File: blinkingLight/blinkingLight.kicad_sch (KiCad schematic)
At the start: 11 parts, among them J1 Conn_02x03_Odd_Even, J2 Conn_01x02_Pin, Q1 BC548, U1 ICM7555xB

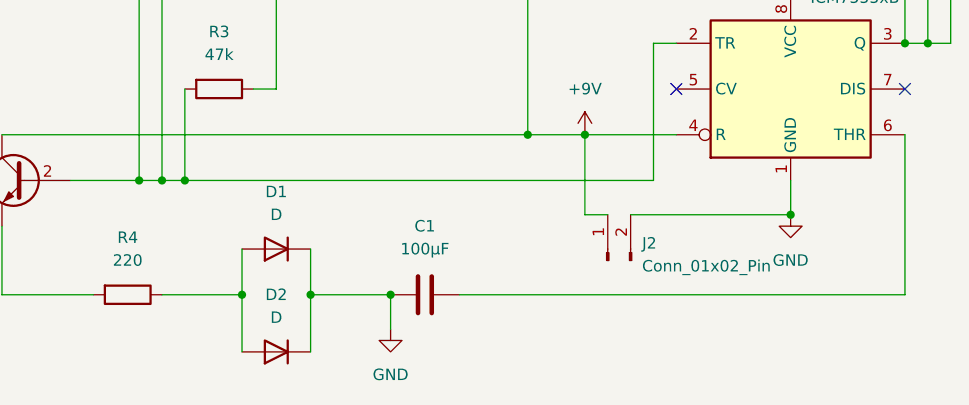
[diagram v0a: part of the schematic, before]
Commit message: push
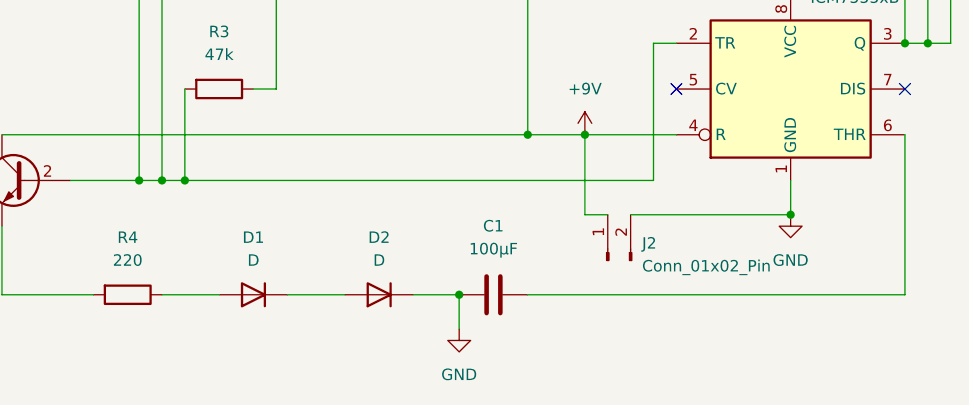
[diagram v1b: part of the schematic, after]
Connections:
- net GND: no longer D1.1 (K)
- net at D1.2 (A), R4.1: no longer D2.2 (A)
- new net: D1.1 (K), D2.2 (A)
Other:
- moved on the sheet: C1, D1, D2
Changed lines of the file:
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@@
 	)
 	(junction
-		(at 96.52 111.76)
-		(diameter 0)
-		(color 0 0 0 0)
-	)
-	(junction
-		(at 104.14 111.76)
+		(at 120.65 111.76)
 		(diameter 0)
 		(color 0 0 0 0)
@@
 	)
 	(junction
-		(at 113.03 111.76)
-		(diameter 0)
-		(color 0 0 0 0)
-	)
-	(junction
 		(at 157.48 102.87)
 		(diameter 0)
@@
 	(wire
 		(pts
-			(xy 104.14 111.76) (xy 104.14 118.11)
-		)
-		(stroke
-			(width 0)
-			(type default)
-		)
-	)
-	(wire
-		(pts
 			(xy 80.01 111.76) (xy 69.85 111.76)
 		)
@@
 	(wire
 		(pts
-			(xy 104.14 111.76) (xy 113.03 111.76)
-		)
-		(stroke
-			(width 0)
-			(type default)
-		)
-	)
-	(wire
-		(pts
 			(xy 77.47 99.06) (xy 85.09 99.06)
 		)
@@
 	(wire
 		(pts
+			(xy 87.63 111.76) (xy 93.98 111.76)
+		)
+		(stroke
+			(width 0)
+			(type default)
+		)
+	)
+	(wire
+		(pts
 			(xy 134.62 102.87) (xy 134.62 93.98)
 		)
@@
 	(wire
 		(pts
-			(xy 96.52 106.68) (xy 96.52 111.76)
+			(xy 115.57 111.76) (xy 120.65 111.76)
 		)
 		(stroke
@@
 	(wire
 		(pts
-			(xy 120.65 111.76) (xy 170.18 111.76)
+			(xy 128.27 111.76) (xy 170.18 111.76)
 		)
 		(stroke
@@
 	(wire
 		(pts
-			(xy 96.52 111.76) (xy 96.52 118.11)
-		)
-		(stroke
-			(width 0)
-			(type default)
-		)
-	)
-	(wire
-		(pts
 			(xy 172.72 69.85) (xy 172.72 83.82)
 		)
@@
 	(wire
 		(pts
-			(xy 113.03 111.76) (xy 113.03 115.57)
+			(xy 120.65 111.76) (xy 120.65 115.57)
+		)
+		(stroke
+			(width 0)
+			(type default)
+		)
+	)
+	(wire
+		(pts
+			(xy 101.6 111.76) (xy 107.95 111.76)
 		)
 		(stroke
@@
 	(wire
 		(pts
-			(xy 96.52 111.76) (xy 87.63 111.76)
-		)
-		(stroke
-			(width 0)
-			(type default)
-		)
-	)
-	(wire
-		(pts
 			(xy 90.17 67.31) (xy 85.09 67.31)
 		)
@@
 		(pts
 			(xy 69.85 111.76) (xy 69.85 104.14)
-		)
-		(stroke
-			(width 0)
-			(type default)
-		)
-	)
-	(wire
-		(pts
-			(xy 104.14 106.68) (xy 104.14 111.76)
 		)
 		(stroke
@@
 	(symbol
 		(lib_id "Device:C")
-		(at 116.84 111.76 270)
+		(at 124.46 111.76 270)
 		(unit 1)
 		(exclude_from_sim no)
@@
 		(fields_autoplaced yes)
 		(property "Reference" "C1"
-			(at 116.84 104.14 90)
+			(at 124.46 104.14 90)
 			(effects
 				(font
@@
 		)
 		(property "Value" "100μF"
-			(at 116.84 106.68 90)
+			(at 124.46 106.68 90)
 			(effects
 				(font
@@
 		)
 		(property "Footprint" "Capacitor_THT:CP_Radial_D8.0mm_P5.00mm"
-			(at 113.03 112.7252 0)
+			(at 120.65 112.7252 0)
 			(effects
 				(font
@@
 		)
 		(property "Datasheet" "~"
-			(at 116.84 111.76 0)
+			(at 124.46 111.76 0)
 			(effects
 				(font
@@
 		)
 		(property "Description" "Unpolarized capacitor"
-			(at 116.84 111.76 0)
+			(at 124.46 111.76 0)
 			(effects
 				(font
@@
 	(symbol
 		(lib_id "Device:D")
-		(at 100.33 118.11 180)
+		(at 111.76 111.76 180)
 		(unit 1)
 		(exclude_from_sim no)
@@
 		(fields_autoplaced yes)
 		(property "Reference" "D2"
-			(at 100.33 111.76 0)
+			(at 111.76 105.41 0)
 			(effects
 				(font
@@
 		)
 		(property "Value" "D"
-			(at 100.33 114.3 0)
+			(at 111.76 107.95 0)
 			(effects
 				(font
@@
 		)
 		(property "Footprint" "LED_THT:LED_D3.0mm_Horizontal_O6.35mm_Z10.0mm"
-			(at 100.33 118.11 0)
+			(at 111.76 111.76 0)
 			(effects
 				(font
@@
 		)
 		(property "Datasheet" "~"
-			(at 100.33 118.11 0)
+			(at 111.76 111.76 0)
 			(effects
 				(font
@@
 		)
 		(property "Description" "Diode"
-			(at 100.33 118.11 0)
+			(at 111.76 111.76 0)
 			(effects
 				(font
@@
 		)
 		(property "Sim.Device" "D"
-			(at 100.33 118.11 0)
+			(at 111.76 111.76 0)
 			(effects
 				(font
@@
 		)
 		(property "Sim.Pins" "1=K 2=A"
-			(at 100.33 118.11 0)
+			(at 111.76 111.76 0)
 			(effects
 				(font
@@
 	(symbol
 		(lib_id "power:GND")
-		(at 113.03 115.57 0)
+		(at 120.65 115.57 0)
 		(unit 1)
 		(exclude_from_sim no)
@@
 		(fields_autoplaced yes)
 		(property "Reference" "#PWR03"
-			(at 113.03 121.92 0)
+			(at 120.65 121.92 0)
 			(effects
 				(font
@@
 		)
 		(property "Value" "GND"
-			(at 113.03 120.65 0)
+			(at 120.65 120.65 0)
 			(effects
 				(font
@@
 		)
 		(property "Footprint" ""
-			(at 113.03 115.57 0)
+			(at 120.65 115.57 0)
 			(effects
 				(font
@@
 		)
 		(property "Datasheet" ""
-			(at 113.03 115.57 0)
+			(at 120.65 115.57 0)
 			(effects
 				(font
@@
 		)
 		(property "Description" "Power symbol creates a global label with name \"GND\" , ground"
-			(at 113.03 115.57 0)
+			(at 120.65 115.57 0)
 			(effects
 				(font
@@
 	(symbol
 		(lib_id "Device:D")
-		(at 100.33 106.68 180)
+		(at 97.79 111.76 180)
 		(unit 1)
 		(exclude_from_sim no)
@@
 		(fields_autoplaced yes)
 		(property "Reference" "D1"
-			(at 100.33 100.33 0)
+			(at 97.79 105.41 0)
 			(effects
 				(font
@@
 		)
 		(property "Value" "D"
-			(at 100.33 102.87 0)
+			(at 97.79 107.95 0)
 			(effects
 				(font
@@
 		)
 		(property "Footprint" "LED_THT:LED_D3.0mm_Horizontal_O6.35mm_Z10.0mm"
-			(at 100.33 106.68 0)
+			(at 97.79 111.76 0)
 			(effects
 				(font
@@
 		)
 		(property "Datasheet" "~"
-			(at 100.33 106.68 0)
+			(at 97.79 111.76 0)
 			(effects
 				(font
@@
 		)
 		(property "Description" "Diode"
-			(at 100.33 106.68 0)
+			(at 97.79 111.76 0)
 			(effects
 				(font
@@
 		)
 		(property "Sim.Device" "D"
-			(at 100.33 106.68 0)
+			(at 97.79 111.76 0)
 			(effects
 				(font
@@
 		)
 		(property "Sim.Pins" "1=K 2=A"
-			(at 100.33 106.68 0)
-			(effects
-				(font
+			(at 97.79 111.76 0)
+			(effects
+				(font

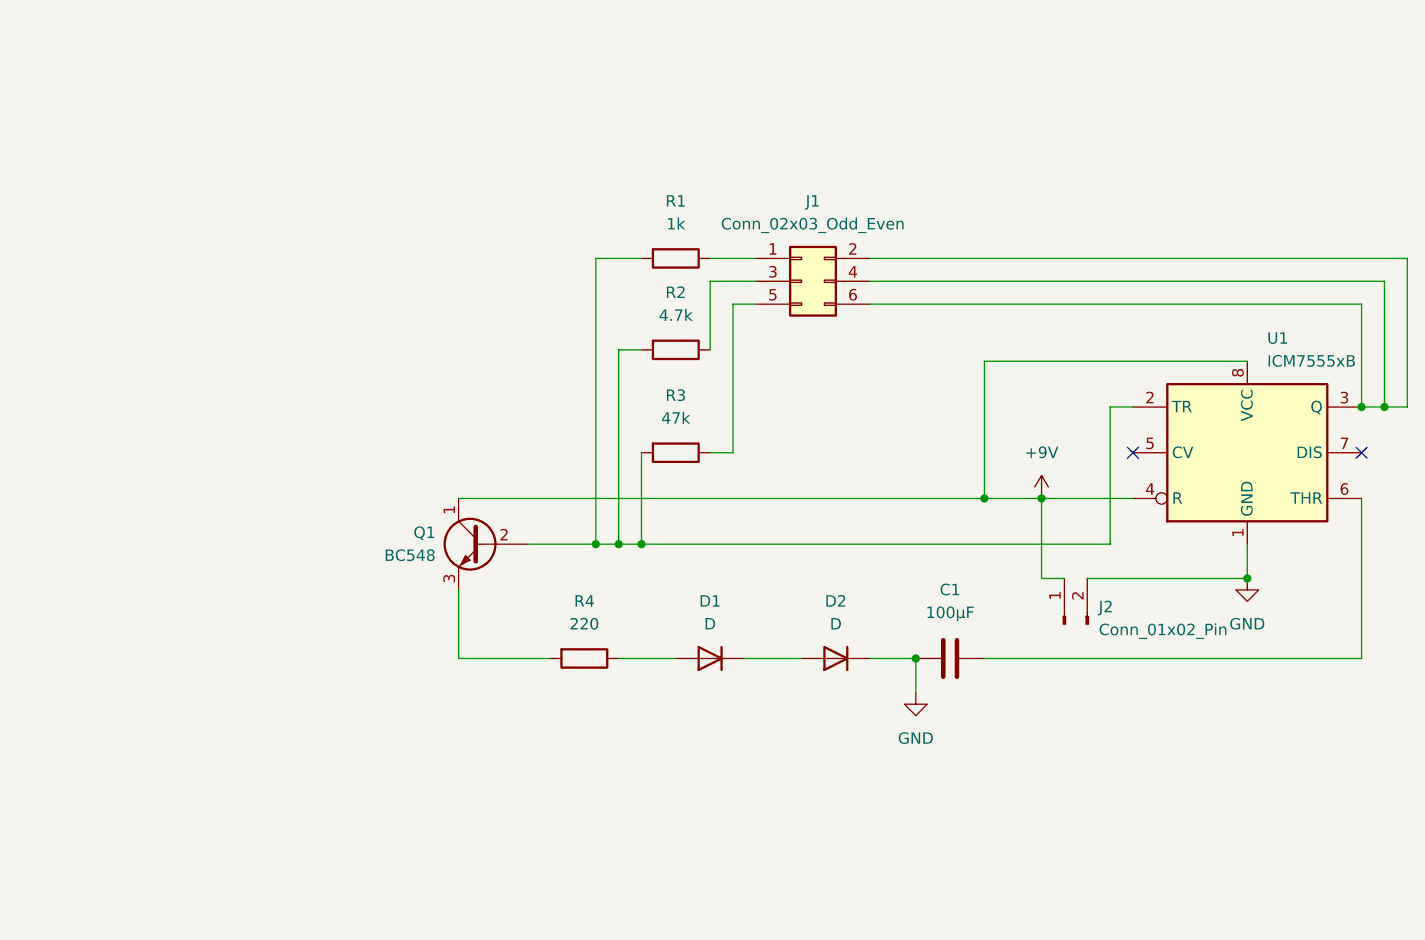
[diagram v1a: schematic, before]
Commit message: push
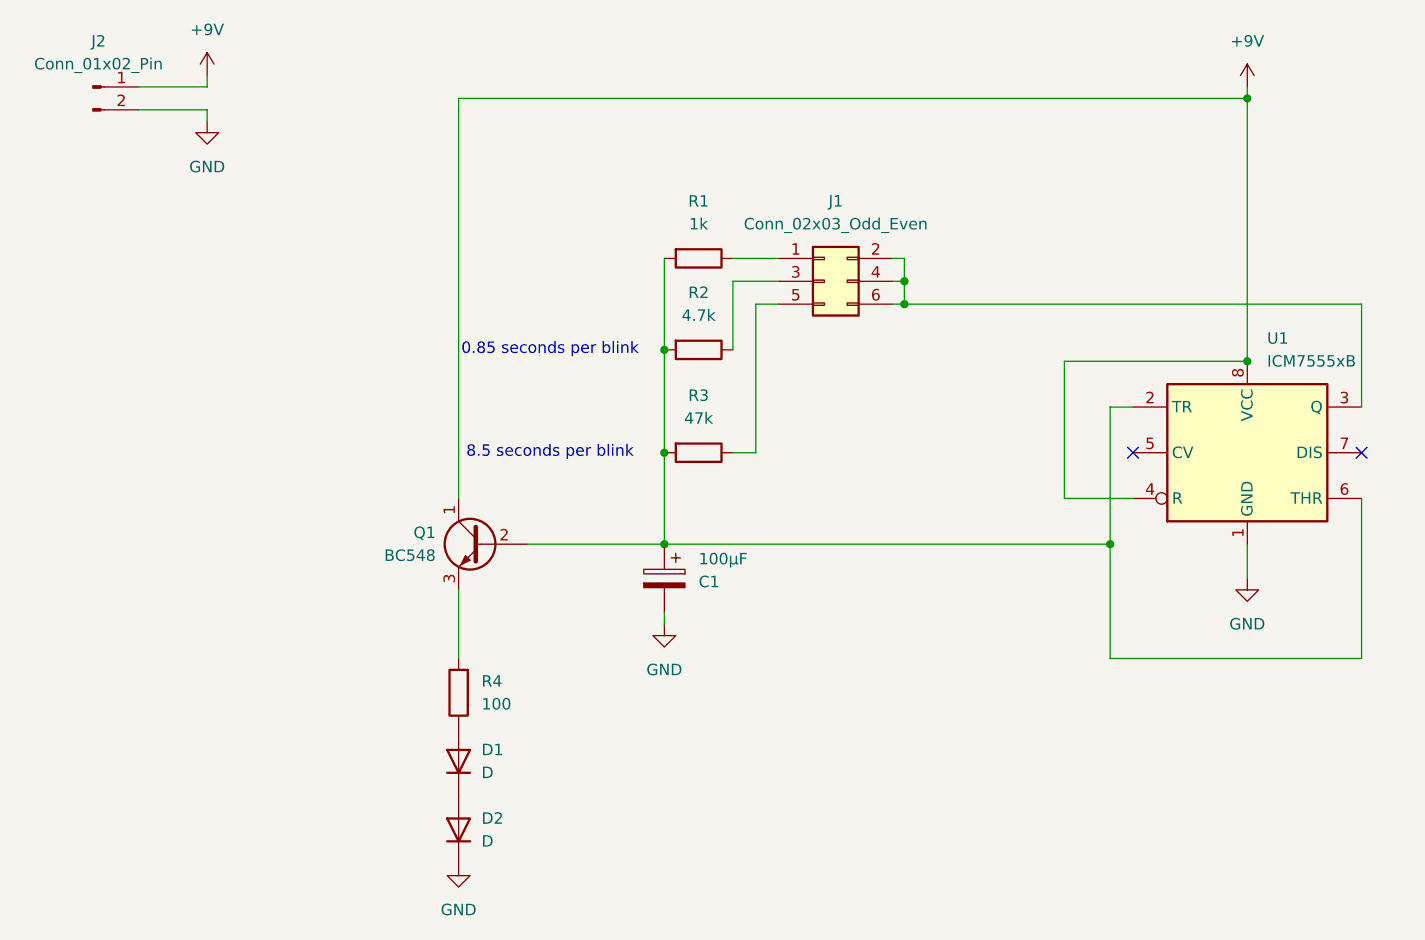
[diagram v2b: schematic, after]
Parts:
- C1: symbol Device:C -> Device:C_Polarized
- R4: value 220 -> 100
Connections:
- net at Q1.2 (B), R1.2, R2.2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: now also C1.1, U1.6 (THR)
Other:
- note added: "0.85 seconds per blink"
- note added: "8.5 seconds per blink"
- moved on the sheet: D1, D2, J1, J2, R1, R2, R3, R4
